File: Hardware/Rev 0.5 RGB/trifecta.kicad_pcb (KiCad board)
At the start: 2 copper layers, 361 x 120.8 mm, 285 parts, among them J1 USB2_C_Receptacle, SW1 SW_Push, SW2 Rotary_Encoder_Switch, SW3 Rotary_Encoder_Switch, SW4 Rotary_Encoder_Switch, U1 ATmega32U4-AU, U2 SRV05-4, Y1 16MHz

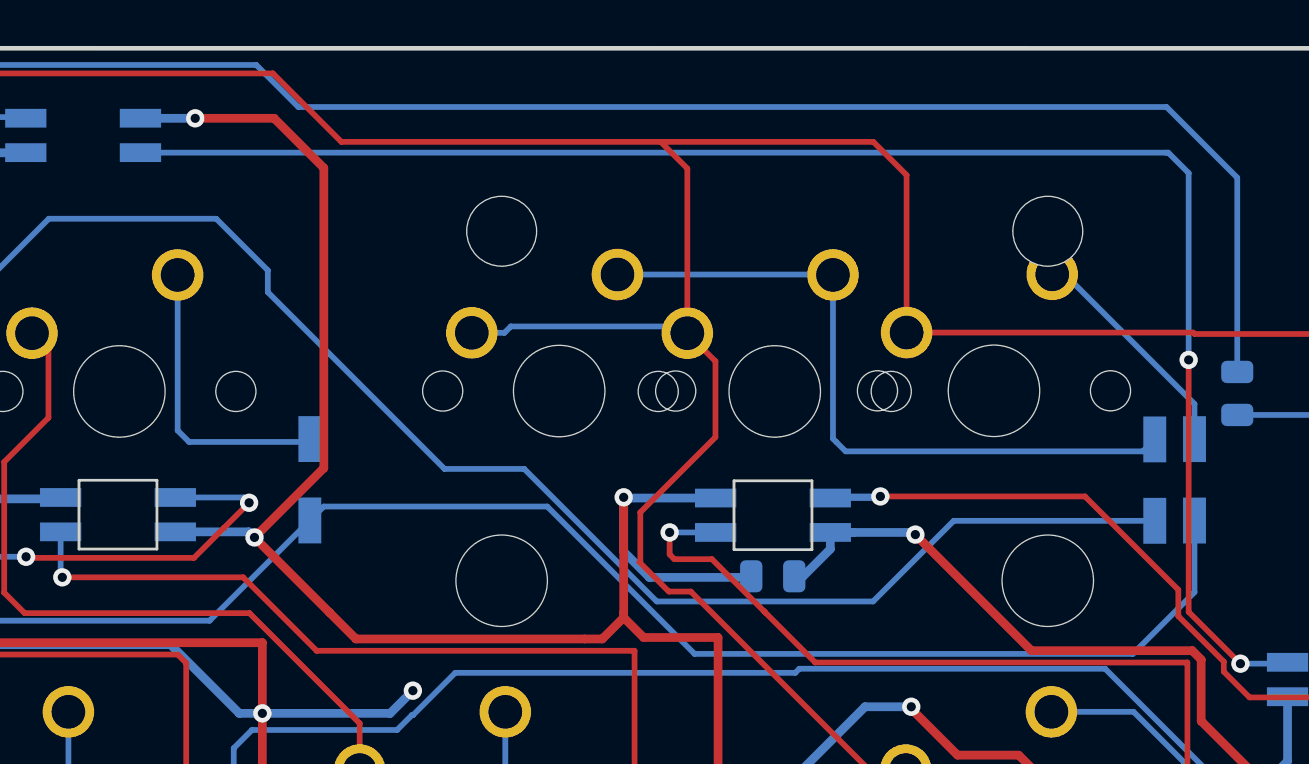
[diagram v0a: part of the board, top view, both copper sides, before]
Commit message: LED37
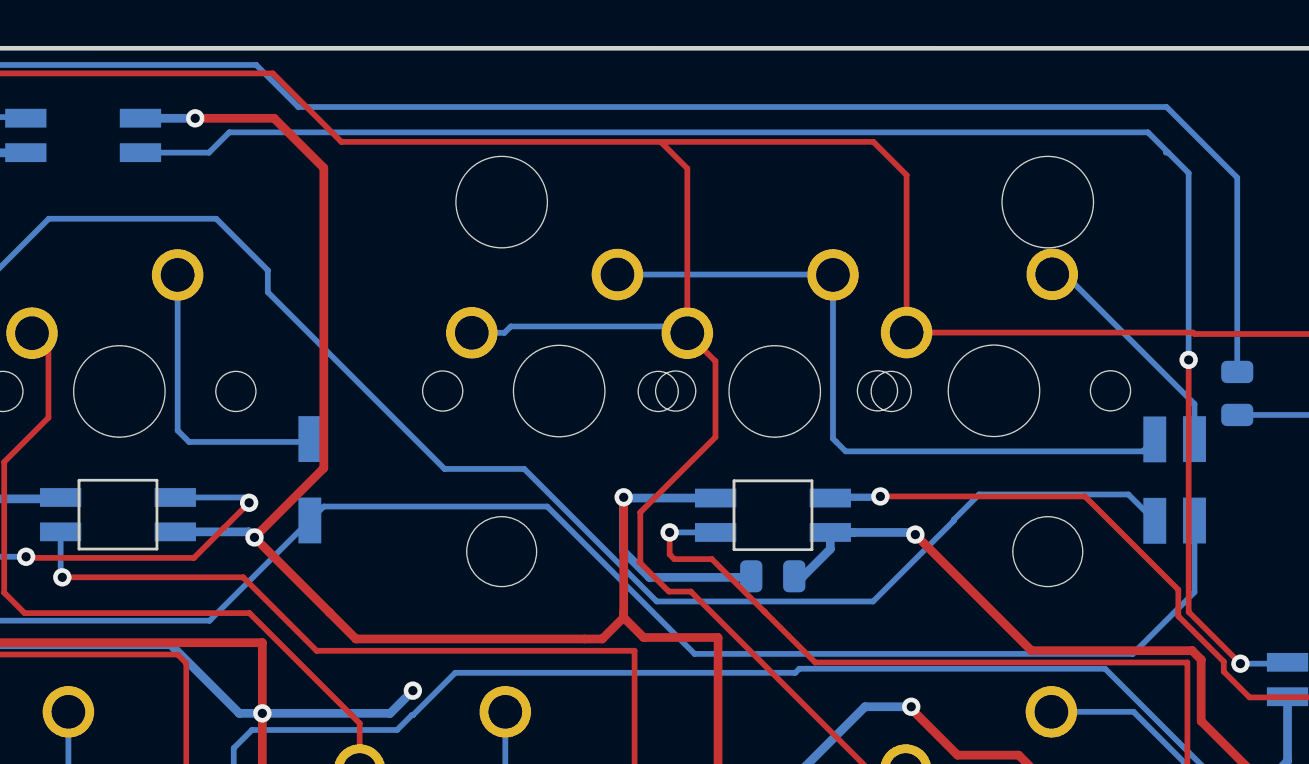
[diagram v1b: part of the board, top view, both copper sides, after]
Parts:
- K_15: footprint MX_Only:MXOnly-2U-NoLED -> MX_Only:MXOnly-2U-ReversedStabilizers-NoLED
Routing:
- net row0: track 372.3 -> 373.3 mm
- net Net-(ULED13-Pad2): track 70.5 -> 71.3 mm
